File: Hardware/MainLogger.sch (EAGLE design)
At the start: 210 parts, among them J3 GEMS_POWER_PLUGINPUT_RT, J4 U.FL, J5 SIM_CDNANO_SF72, Q1 DMG3404, Q2 MOSFET_PCH-DMP3036SFG, Q3 MOSFET_PCH-DMP3036SFG, Q4 DMG3404, Q5 NX2301P, Q6 NX2301P, U1 FXMAR2102UMLP, U10 SN74AUP3G34DCU, U11 TCK111G, U12 LTC4412S6, U13 TCR2LE31ESV, U14 LP59073.3VYKE, U15 MIC22602, U16 BQ25616, U17 TPS61282D, U18 MCP23018QFN, U19 MCP23018QFN, U2 VEML3328, U20 MAX-M8W, U21 MCP79412SOIC, U22 HALL_EFFECT_SI7201, U23 PCA9634QFN, U24 SN74LVC1G17DCK, U25 TPL5010DDC, U26 TPL5010DDC, U27 MB85RC, U28 FXMAR2102UMLP, U29 SIT1552, U3 MMC5633, U30 TCK111G, U31 FPF2195BUCX, U4 MXC6655, U5 PAC1934QFN, U6 PAC1934QFN, U7 SHT40, U8 SN74AUP1G08DCK, U9 FXMAR2102UMLP

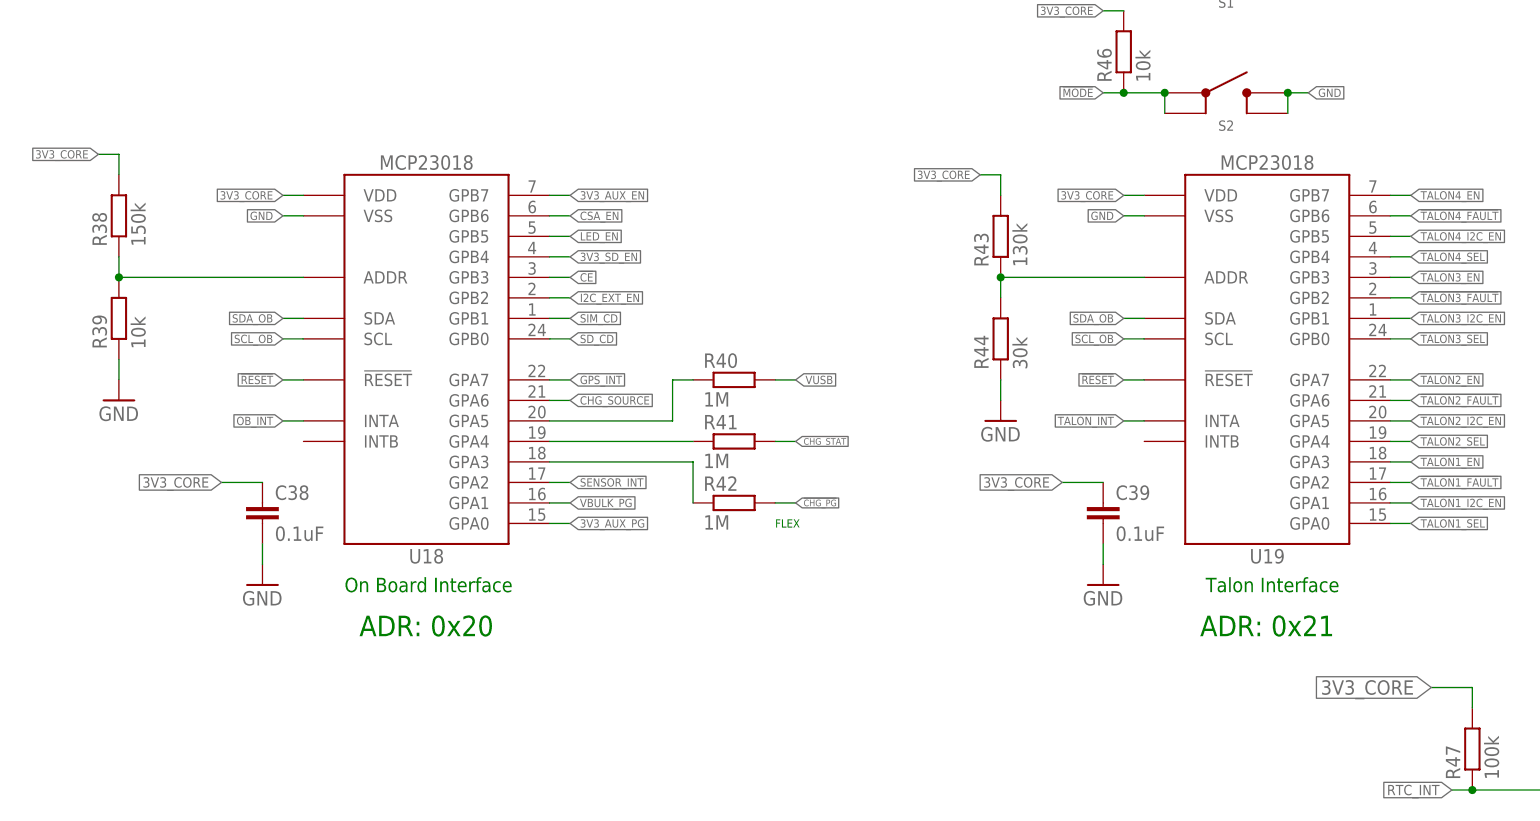
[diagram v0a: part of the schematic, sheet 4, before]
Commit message: v1.5 Update
Updated schematic and layout, boards sent to fab
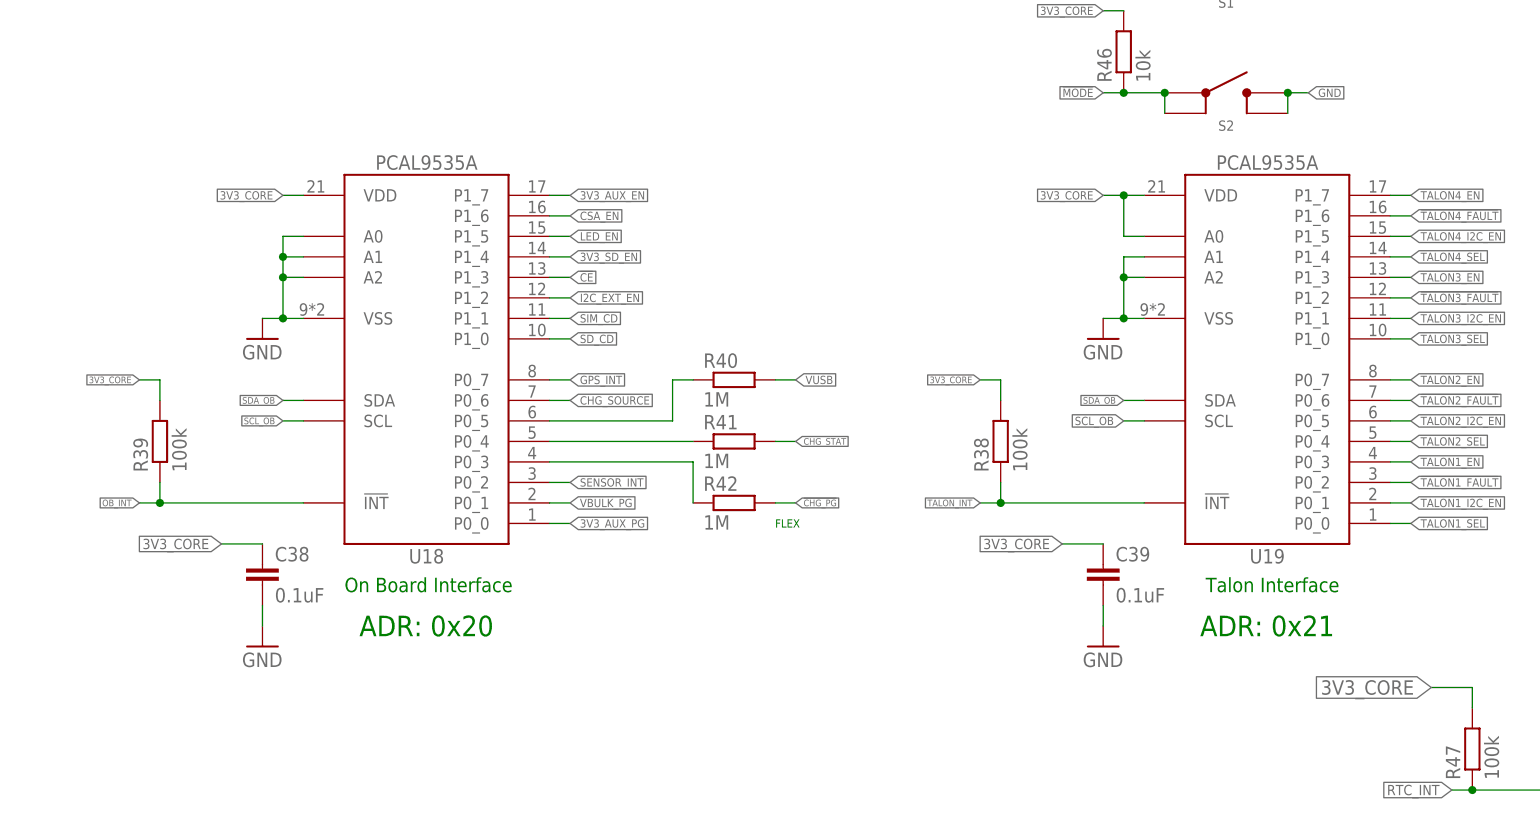
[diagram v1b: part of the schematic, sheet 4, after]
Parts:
- removed R43: 130k, bschulz_passives:R-EU_130KR0402
- removed R44: 30k, bschulz_passives:R-EU_30KR0402
- R38: value 150k -> 100k; device bschulz_passives:R-EU_150KR0402 -> bschulz_passives:R-EU_100KR0402
- R39: value 10k -> 100k; device bschulz_passives:R-EU_10KR0402 -> bschulz_passives:R-EU_100KR0402
- U18, U19: value MCP23018QFN -> PCAL9535AQFN; device bschulz:MCP23018QFN -> bschulz:PCAL9535AQFN
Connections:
- removed net N$35: R43.1, R44.2, U19.ADDR
- removed net N$38: R38.1, R39.2, U18.ADDR
- net !CE: now also U18.P1_3; no longer U18.GPB3
- net !RESET: no longer U18.!RESET, U19.!RESET
- net !TALON1_FAULT: now also U19.P0_2; no longer U19.GPA2
- net !TALON2_FAULT: now also U19.P0_6; no longer U19.GPA6
- net !TALON3_FAULT: now also U19.P1_2; no longer U19.GPB2
- net !TALON4_FAULT: now also U19.P1_6; no longer U19.GPB6
- net 3V3_AUX_EN: now also U18.P1_7; no longer U18.GPB7
- net 3V3_AUX_PG: now also U18.P0_0; no longer U18.GPA0
- net 3V3_CORE: now also R39.2, U19.A0; no longer R43.2
- net 3V3_SD_EN: now also U18.P1_4; no longer U18.GPB4
- net CHG_SOURCE: now also U18.P0_6; no longer U18.GPA6
- net CSA_EN: now also U18.P1_6; no longer U18.GPB6
- net GND: now also U18.A0, U18.A1, U18.A2, U19.A1, U19.A2; no longer R39.1, R44.1
- net GPS_INT: now also U18.P0_7; no longer U18.GPA7
- net I2C_EXT_EN: now also U18.P1_2; no longer U18.GPB2
- net LED_EN: now also U18.P1_5; no longer U18.GPB5
- net N$6: now also U18.P0_4; no longer U18.GPA4
- net N$8: now also U18.P0_5; no longer U18.GPA5
- net N$9: now also U18.P0_3; no longer U18.GPA3
- net OB_INT: now also R39.1, U18.!INT; no longer U18.INTA
- net SD_CD: now also U18.P1_0; no longer U18.GPB0
- net SENSOR_INT: now also U18.P0_2; no longer U18.GPA2
- net SIM_CD: now also U18.P1_1; no longer U18.GPB1
- net TALON1_EN: now also U19.P0_3; no longer U19.GPA3
- net TALON1_I2C_EN: now also U19.P0_1; no longer U19.GPA1
- net TALON1_SEL: now also U19.P0_0; no longer U19.GPA0
- net TALON2_EN: now also U19.P0_7; no longer U19.GPA7
- net TALON2_I2C_EN: now also U19.P0_5; no longer U19.GPA5
- net TALON2_SEL: now also U19.P0_4; no longer U19.GPA4
- net TALON3_EN: now also U19.P1_3; no longer U19.GPB3
- net TALON3_I2C_EN: now also U19.P1_1; no longer U19.GPB1
- net TALON3_SEL: now also U19.P1_0; no longer U19.GPB0
- net TALON4_EN: now also U19.P1_7; no longer U19.GPB7
- net TALON4_I2C_EN: now also U19.P1_5; no longer U19.GPB5
- net TALON4_SEL: now also U19.P1_4; no longer U19.GPB4
- net TALON_INT: now also R38.1, U19.!INT; no longer U19.INTA
- net VBULK_PG: now also U18.P0_1; no longer U18.GPA1
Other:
- moved on the sheet: C38, C39, R38, R39
